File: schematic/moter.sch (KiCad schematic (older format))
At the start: 10 parts, among them J10 Conn_01x04_Male, J11 Conn_01x04_Male, J8 Conn_01x04_Male, J9 Conn_01x08_Male, U3 PCA9685PW

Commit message: added LSM6DSOX and LIS2MDL for IMU
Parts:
- removed J10, J11, J8: Conn_01x04_Male, Connector_PinHeader_2.54mm:PinHeader_1x04_P2.54mm_Vertical, symbol Connector:Conn_01x04_Male
- added J8: Conn_01x05, Connector_JST:JST_XH_B5B-XH-A_1x05_P2.50mm_Vertical, symbol Connector_Generic:Conn_01x05
- J9: footprint Connector_PinHeader_2.54mm:PinHeader_1x08_P2.54mm_Vertical -> Connector_JST:JST_XH_B8B-XH-A_1x08_P2.50mm_Vertical
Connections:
- net labels removed: +5V
- wire segments 33 -> 26
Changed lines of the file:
@@
 	0    1    1    0
-$EndComp
-$Comp
-L Connector:Conn_01x04_Male J?
-U 1 1 5EF64F3D
-P 4850 1950
-AR Path="/5EF64F3D" Ref="J?"  Part="1"
-AR Path="/5EF07089/5EF64F3D" Ref="J8"  Part="1"
-F 0 "J8" H 4958 2231 50  0000 C CNN
-F 1 "Conn_01x04_Male" H 4958 2140 50  0000 C CNN
-F 2 "Connector_PinHeader_2.54mm:PinHeader_1x04_P2.54mm_Vertical" H 4850 1950 50  0001 C CNN
-F 3 "~" H 4850 1950 50  0001 C CNN
-	1    4850 1950
-	1    0    0    -1
 $EndComp
 Text GLabel 5050 1850 2    50   Input ~ 0
@@
 F 0 "J9" H 4958 3231 50  0000 C CNN
 F 1 "Conn_01x08_Male" H 4958 3140 50  0000 C CNN
-F 2 "Connector_PinHeader_2.54mm:PinHeader_1x08_P2.54mm_Vertical" H 4850 2750 50  0001 C CNN
+F 2 "Connector_JST:JST_XH_B8B-XH-A_1x08_P2.50mm_Vertical" H 4850 2750 50  0001 C CNN
 F 3 "~" H 4850 2750 50  0001 C CNN
 	1    4850 2750
@@
 	6050 2950 6800 2950
 $Comp
-L Connector:Conn_01x04_Male J?
-U 1 1 5EF64F90
-P 6150 1900
-AR Path="/5EF64F90" Ref="J?"  Part="1"
-AR Path="/5EF07089/5EF64F90" Ref="J10"  Part="1"
-F 0 "J10" H 6258 2181 50  0000 C CNN
-F 1 "Conn_01x04_Male" H 6258 2090 50  0000 C CNN
-F 2 "Connector_PinHeader_2.54mm:PinHeader_1x04_P2.54mm_Vertical" H 6150 1900 50  0001 C CNN
-F 3 "~" H 6150 1900 50  0001 C CNN
-	1    6150 1900
-	1    0    0    -1
-$EndComp
-$Comp
-L Connector:Conn_01x04_Male J?
-U 1 1 5EF64F96
-P 7000 1900
-AR Path="/5EF64F96" Ref="J?"  Part="1"
-AR Path="/5EF07089/5EF64F96" Ref="J11"  Part="1"
-F 0 "J11" H 7108 2181 50  0000 C CNN
-F 1 "Conn_01x04_Male" H 7108 2090 50  0000 C CNN
-F 2 "Connector_PinHeader_2.54mm:PinHeader_1x04_P2.54mm_Vertical" H 7000 1900 50  0001 C CNN
-F 3 "~" H 7000 1900 50  0001 C CNN
-	1    7000 1900
-	1    0    0    -1
+L Connector_Generic:Conn_01x05 J8
+U 1 1 5ED5189E
+P 4850 1950
+F 0 "J8" H 4768 1525 50  0000 C CNN
+F 1 "Conn_01x05" H 4768 1616 50  0000 C CNN
+F 2 "Connector_JST:JST_XH_B5B-XH-A_1x05_P2.50mm_Vertical" H 4850 1950 50  0001 C CNN
+F 3 "~" H 4850 1950 50  0001 C CNN
+	1    4850 1950
+	-1   0    0    1
 $EndComp
 $Comp
 L power:GND #PWR?
-U 1 1 5EF64F9C
-P 7200 2100
-AR Path="/5EF64F9C" Ref="#PWR?"  Part="1"
-AR Path="/5EF07089/5EF64F9C" Ref="#PWR036"  Part="1"
-F 0 "#PWR036" H 7200 1850 50  0001 C CNN
-F 1 "GND" H 7205 1927 50  0000 C CNN
-F 2 "" H 7200 2100 50  0001 C CNN
-F 3 "" H 7200 2100 50  0001 C CNN
-	1    7200 2100
-	1    0    0    -1
+U 1 1 5ED56EC8
+P 5050 1750
+AR Path="/5ED56EC8" Ref="#PWR?"  Part="1"
+AR Path="/5EF07089/5ED56EC8" Ref="#PWR0101"  Part="1"
+F 0 "#PWR0101" H 5050 1500 50  0001 C CNN
+F 1 "GND" V 5055 1577 50  0000 C CNN
+F 2 "" H 5050 1750 50  0001 C CNN
+F 3 "" H 5050 1750 50  0001 C CNN
+	1    5050 1750
+	0    -1   -1   0
 $EndComp
-Wire Wire Line
-	7200 2150 7200 2100
-Connection ~ 7200 2100
-Wire Wire Line
-	7200 2100 7200 2000
-Wire Wire Line
-	7200 2000 7200 1900
-Connection ~ 7200 2000
-Wire Wire Line
-	7200 1900 7200 1800
-Connection ~ 7200 1900
-$Comp
-L power:+5V #PWR?
-U 1 1 5EF64FA9
-P 6350 2100
-AR Path="/5EF64FA9" Ref="#PWR?"  Part="1"
-AR Path="/5EF07089/5EF64FA9" Ref="#PWR035"  Part="1"
-F 0 "#PWR035" H 6350 1950 50  0001 C CNN
-F 1 "+5V" H 6365 2273 50  0000 C CNN
-F 2 "" H 6350 2100 50  0001 C CNN
-F 3 "" H 6350 2100 50  0001 C CNN
-	1    6350 2100
-	-1   0    0    1
-$EndComp
-Wire Wire Line
-	6350 2100 6350 2000
-Connection ~ 6350 2100
-Wire Wire Line
-	6350 2000 6350 1900
-Connection ~ 6350 2000
-Wire Wire Line
-	6350 1900 6350 1800
-Connection ~ 6350 1900
 $EndSCHEMATC

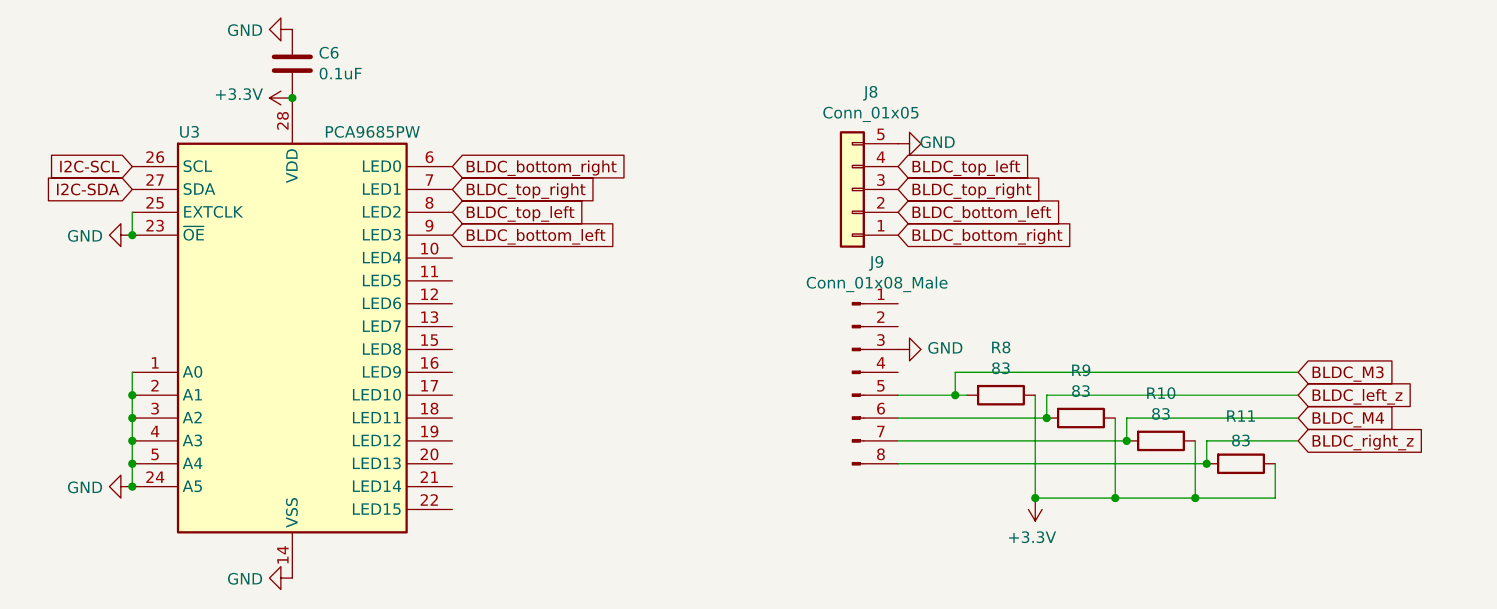
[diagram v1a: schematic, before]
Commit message: new pcb design
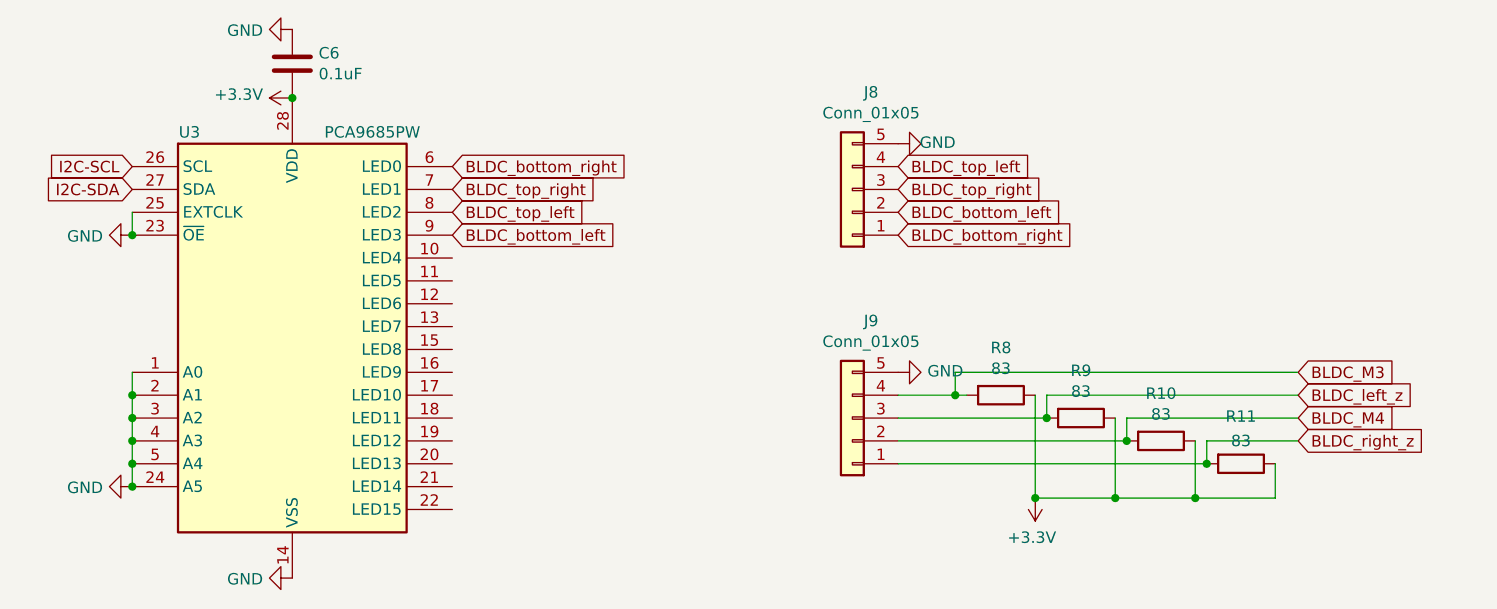
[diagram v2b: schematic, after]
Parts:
- removed J9: Conn_01x08_Male, Connector_JST:JST_XH_B8B-XH-A_1x08_P2.50mm_Vertical, symbol Connector:Conn_01x08_Male
- added J9: Conn_01x05, Connector_JST:JST_XH_B5B-XH-A_1x05_P2.50mm_Vertical, symbol Connector_Generic:Conn_01x05
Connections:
- net BLDC_M3: now also J9.4 (Pin_4)
- net BLDC_M4: now also J9.2 (Pin_2)
- net BLDC_left_z: now also J9.3 (Pin_3)
- net BLDC_right_z: now also J9.1 (Pin_1)
- net GND: now also J9.5 (Pin_5)
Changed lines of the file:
@@
 BLDC_bottom_right
-$Comp
-L Connector:Conn_01x08_Male J?
-U 1 1 5EF64F47
-P 4850 2750
-AR Path="/5EF64F47" Ref="J?"  Part="1"
-AR Path="/5EF07089/5EF64F47" Ref="J9"  Part="1"
-F 0 "J9" H 4958 3231 50  0000 C CNN
-F 1 "Conn_01x08_Male" H 4958 3140 50  0000 C CNN
-F 2 "Connector_JST:JST_XH_B8B-XH-A_1x08_P2.50mm_Vertical" H 4850 2750 50  0001 C CNN
-F 3 "~" H 4850 2750 50  0001 C CNN
-	1    4850 2750
-	1    0    0    -1
-$EndComp
 $Comp
 L power:GND #PWR?
 U 1 1 5EF64F4D
-P 5050 2650
+P 5050 2750
 AR Path="/5EF64F4D" Ref="#PWR?"  Part="1"
 AR Path="/5EF07089/5EF64F4D" Ref="#PWR033"  Part="1"
-F 0 "#PWR033" H 5050 2400 50  0001 C CNN
-F 1 "GND" V 5055 2522 50  0000 R CNN
-F 2 "" H 5050 2650 50  0001 C CNN
-F 3 "" H 5050 2650 50  0001 C CNN
-	1    5050 2650
+F 0 "#PWR033" H 5050 2500 50  0001 C CNN
+F 1 "GND" V 5055 2622 50  0000 R CNN
+F 2 "" H 5050 2750 50  0001 C CNN
+F 3 "" H 5050 2750 50  0001 C CNN
+	1    5050 2750
 	0    -1   -1   0
 $EndComp
@@
 	0    -1   -1   0
 $EndComp
+$Comp
+L Connector_Generic:Conn_01x05 J9
+U 1 1 5EE5CFE9
+P 4850 2950
+F 0 "J9" H 4768 2525 50  0000 C CNN
+F 1 "Conn_01x05" H 4768 2616 50  0000 C CNN
+F 2 "Connector_JST:JST_XH_B5B-XH-A_1x05_P2.50mm_Vertical" H 4850 2950 50  0001 C CNN
+F 3 "~" H 4850 2950 50  0001 C CNN
+	1    4850 2950
+	-1   0    0    1
+$EndComp
 $EndSCHEMATC
